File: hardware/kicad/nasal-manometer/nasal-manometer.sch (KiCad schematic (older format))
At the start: 12 parts, among them J1 Vout, J2 Vref

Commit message: Schematic updated
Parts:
- R2, R3: footprint (none) -> Resistor_SMD:R_0805_2012Metric
- Rg: footprint (none) -> Resistor_SMD:R_0603_1608Metric
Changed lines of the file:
@@
 $EndComp
 $Comp
-L power:GND #PWR?
+L power:GND #PWR0101
 U 1 1 5CD492E7
 P 5850 3725
-F 0 "#PWR?" H 5850 3475 50  0001 C CNN
+F 0 "#PWR0101" H 5850 3475 50  0001 C CNN
 F 1 "GND" H 5855 3552 50  0000 C CNN
 F 2 "" H 5850 3725 50  0001 C CNN
@@
 $EndComp
 $Comp
-L power:GND #PWR?
+L power:GND #PWR0102
 U 1 1 5CD4A19E
 P 4525 2825
-F 0 "#PWR?" H 4525 2575 50  0001 C CNN
+F 0 "#PWR0102" H 4525 2575 50  0001 C CNN
 F 1 "GND" H 4530 2652 50  0000 C CNN
 F 2 "" H 4525 2825 50  0001 C CNN
@@
 $EndComp
 $Comp
-L power:+5V #PWR?
+L power:+5V #PWR0103
 U 1 1 5CD4A7C1
 P 4525 2225
-F 0 "#PWR?" H 4525 2075 50  0001 C CNN
+F 0 "#PWR0103" H 4525 2075 50  0001 C CNN
 F 1 "+5V" H 4540 2398 50  0000 C CNN
 F 2 "" H 4525 2225 50  0001 C CNN
@@
 $EndComp
 $Comp
-L power:GND #PWR?
+L power:GND #PWR0104
 U 1 1 5CD5646F
 P 3650 2725
-F 0 "#PWR?" H 3650 2475 50  0001 C CNN
+F 0 "#PWR0104" H 3650 2475 50  0001 C CNN
 F 1 "GND" H 3655 2552 50  0000 C CNN
 F 2 "" H 3650 2725 50  0001 C CNN
@@
 $EndComp
 $Comp
-L power:GND #PWR?
+L power:GND #PWR0105
 U 1 1 5CD56C7C
 P 3900 2725
-F 0 "#PWR?" H 3900 2475 50  0001 C CNN
+F 0 "#PWR0105" H 3900 2475 50  0001 C CNN
 F 1 "GND" H 3905 2552 50  0000 C CNN
 F 2 "" H 3900 2725 50  0001 C CNN
@@
 Connection ~ 3650 2425
 $Comp
-L power:+5V #PWR?
+L power:+5V #PWR0106
 U 1 1 5CD5BB98
 P 3650 2025
-F 0 "#PWR?" H 3650 1875 50  0001 C CNN
+F 0 "#PWR0106" H 3650 1875 50  0001 C CNN
 F 1 "+5V" H 3665 2198 50  0000 C CNN
 F 2 "" H 3650 2025 50  0001 C CNN
@@
 F 0 "R2" H 4270 4321 50  0000 L CNN
 F 1 "10 KOhm" H 4270 4230 50  0000 L CNN
-F 2 "" V 4130 4275 50  0001 C CNN
+F 2 "Resistor_SMD:R_0805_2012Metric" V 4130 4275 50  0001 C CNN
 F 3 "~" H 4200 4275 50  0001 C CNN
 	1    4200 4275
@@
 F 0 "R3" H 4270 5021 50  0000 L CNN
 F 1 "15 KOhm" H 4270 4930 50  0000 L CNN
-F 2 "" V 4130 4975 50  0001 C CNN
+F 2 "Resistor_SMD:R_0805_2012Metric" V 4130 4975 50  0001 C CNN
 F 3 "~" H 4200 4975 50  0001 C CNN
 	1    4200 4975
@@
 	4200 2425 4325 2425
 $Comp
-L power:GND #PWR?
+L power:GND #PWR0107
 U 1 1 5CD3B5F1
 P 4200 5125
-F 0 "#PWR?" H 4200 4875 50  0001 C CNN
+F 0 "#PWR0107" H 4200 4875 50  0001 C CNN
 F 1 "GND" H 4205 4952 50  0000 C CNN
 F 2 "" H 4200 5125 50  0001 C CNN
@@
 	4200 4650 4200 4825
 $Comp
-L power:GND #PWR?
+L power:GND #PWR0108
 U 1 1 5CD3F60A
 P 4950 5050
-F 0 "#PWR?" H 4950 4800 50  0001 C CNN
+F 0 "#PWR0108" H 4950 4800 50  0001 C CNN
 F 1 "GND" H 4955 4877 50  0000 C CNN
 F 2 "" H 4950 5050 50  0001 C CNN
@@
 	5350 5325 5350 4750
 $Comp
-L power:+5V #PWR?
+L power:+5V #PWR0109
 U 1 1 5CD41D10
 P 4950 4450
-F 0 "#PWR?" H 4950 4300 50  0001 C CNN
+F 0 "#PWR0109" H 4950 4300 50  0001 C CNN
 F 1 "+5V" H 4965 4623 50  0000 C CNN
 F 2 "" H 4950 4450 50  0001 C CNN
@@
 Connection ~ 5350 4750
 $Comp
-L power:GND #PWR?
+L power:GND #PWR0110
 U 1 1 5CD4D2C8
 P 7125 4525
-F 0 "#PWR?" H 7125 4275 50  0001 C CNN
+F 0 "#PWR0110" H 7125 4275 50  0001 C CNN
 F 1 "GND" H 7130 4352 50  0000 C CNN
 F 2 "" H 7125 4525 50  0001 C CNN
@@
 $EndComp
 $Comp
-L power:+5V #PWR?
+L power:+5V #PWR0111
 U 1 1 5CD4D986
 P 7125 3925
-F 0 "#PWR?" H 7125 3775 50  0001 C CNN
+F 0 "#PWR0111" H 7125 3775 50  0001 C CNN
 F 1 "+5V" H 7140 4098 50  0000 C CNN
 F 2 "" H 7125 3925 50  0001 C CNN
@@
 F 0 "Rg" H 6600 4275 50  0000 L CNN
 F 1 "500 Ohm" H 6350 4175 50  0000 L CNN
-F 2 "" V 6680 4225 50  0001 C CNN
+F 2 "Resistor_SMD:R_0603_1608Metric" V 6680 4225 50  0001 C CNN
 F 3 "~" H 6750 4225 50  0001 C CNN
 	1    6750 4225

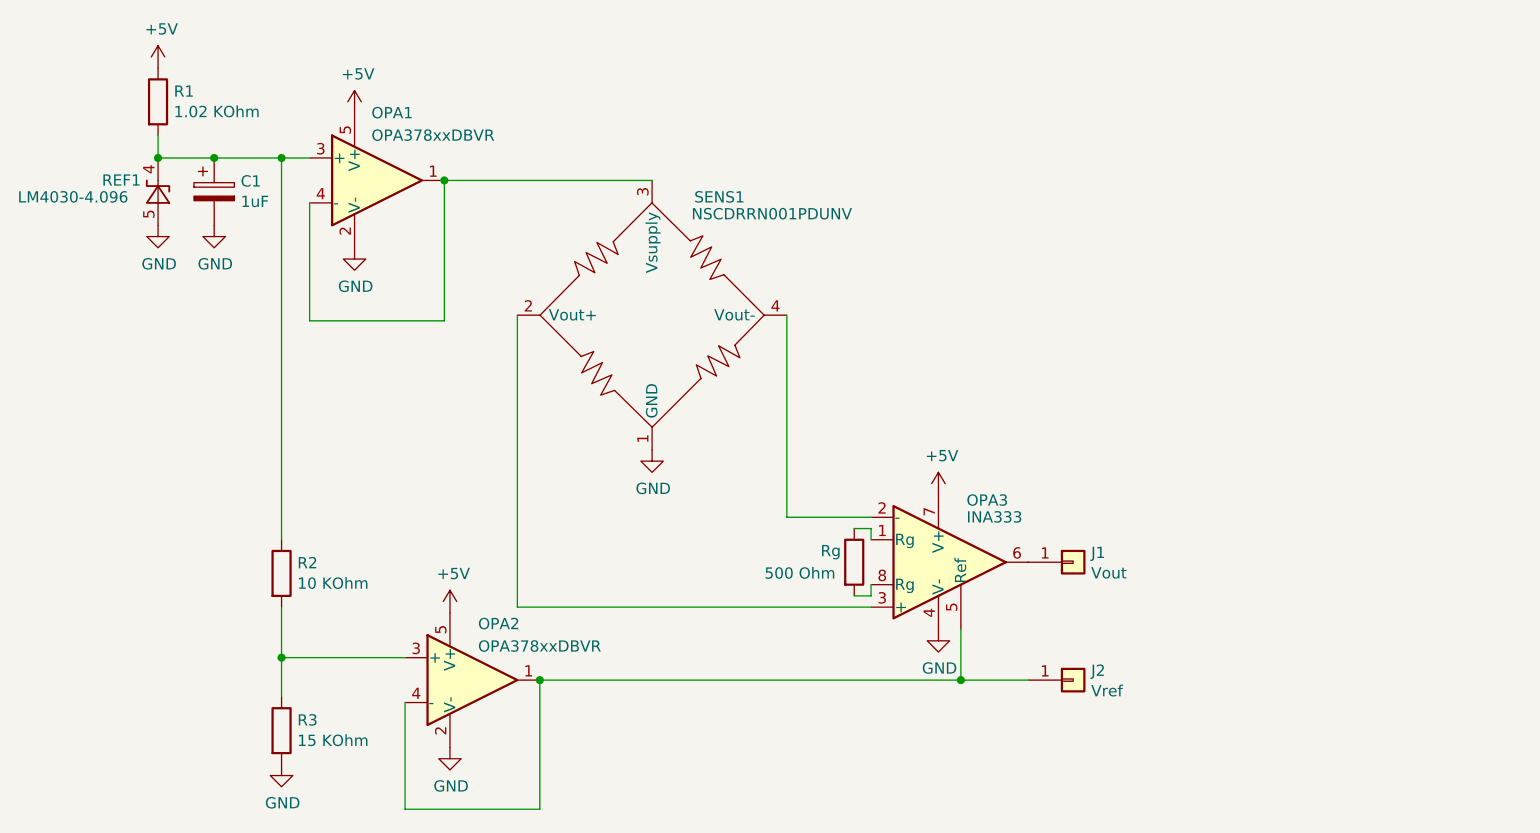
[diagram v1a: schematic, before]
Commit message: Building the board
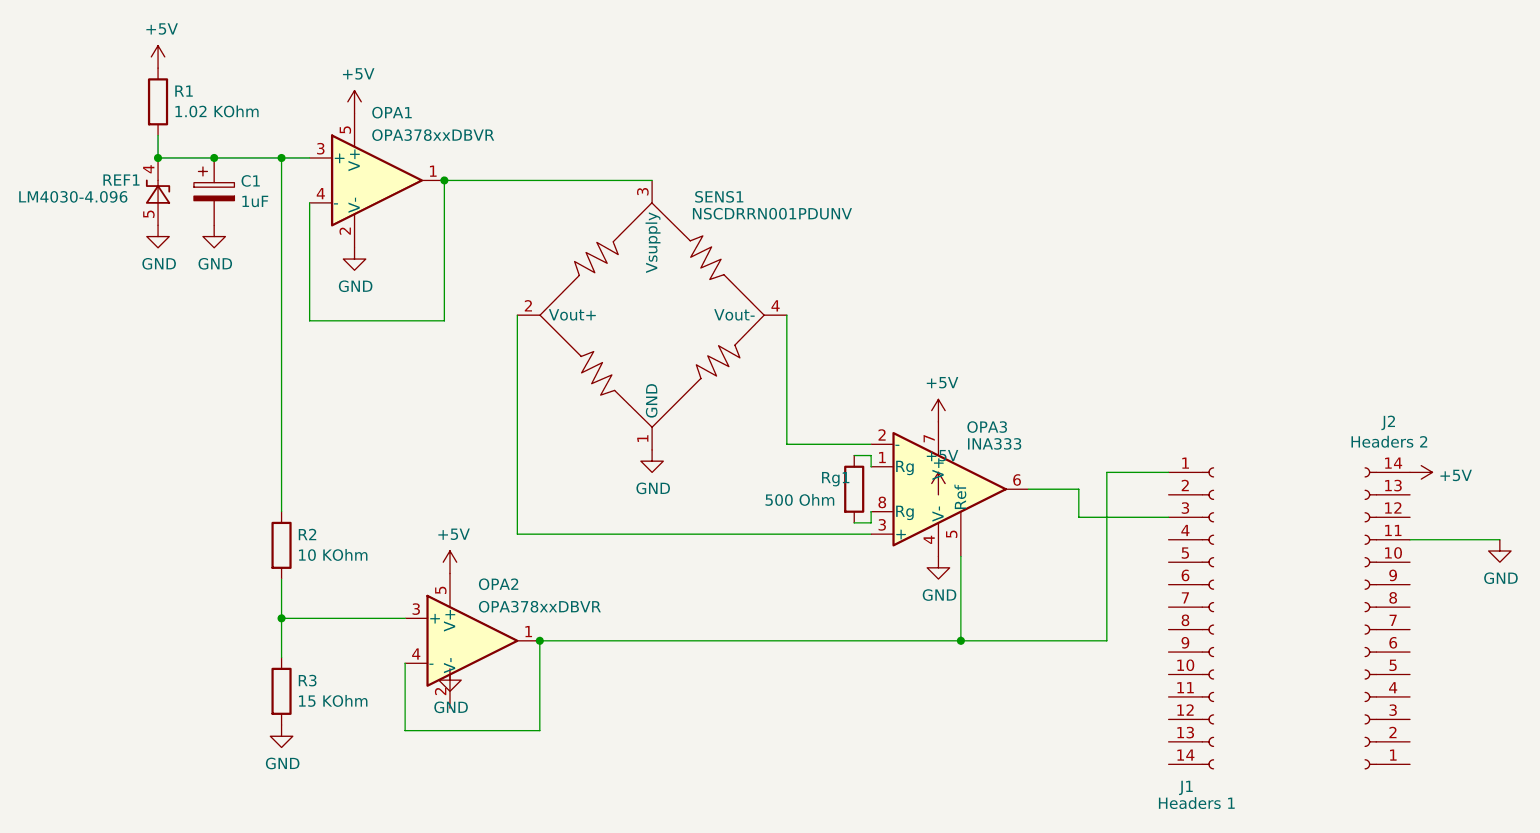
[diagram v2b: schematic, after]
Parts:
- removed J1: Vout, symbol Connector_Generic:Conn_01x01
- removed J2: Vref, symbol Connector_Generic:Conn_01x01
- added J1: Headers 1, Connector_PinSocket_2.54mm:PinSocket_1x14_P2.54mm_Vertical, symbol Connector:Conn_01x14_Female
- added J2: Headers 2, Connector_PinSocket_2.54mm:PinSocket_1x14_P2.54mm_Vertical, symbol Connector:Conn_01x14_Female
- renumbered Rg to Rg1
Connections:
- net +5V: now also J2.14 (Pin_14)
- net GND: now also J2.11 (Pin_11); no longer OPA2.2 (V-)
- net at OPA2.1, OPA2.4 (-), OPA3.5 (Ref): now also J1.1 (Pin_1)
- net at OPA3.6: now also J1.3 (Pin_3)
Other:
- moved on the sheet: OPA2, OPA3, R2, R3, Rg1
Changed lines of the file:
@@
 L Device:R R2
 U 1 1 5CD37D29
-P 4200 4275
-F 0 "R2" H 4270 4321 50  0000 L CNN
-F 1 "10 KOhm" H 4270 4230 50  0000 L CNN
-F 2 "Resistor_SMD:R_0805_2012Metric" V 4130 4275 50  0001 C CNN
-F 3 "~" H 4200 4275 50  0001 C CNN
-	1    4200 4275
+P 4200 4150
+F 0 "R2" H 4270 4196 50  0000 L CNN
+F 1 "10 KOhm" H 4270 4105 50  0000 L CNN
+F 2 "Resistor_SMD:R_0805_2012Metric" V 4130 4150 50  0001 C CNN
+F 3 "~" H 4200 4150 50  0001 C CNN
+	1    4200 4150
 	1    0    0    -1
 $EndComp
@@
 L Device:R R3
 U 1 1 5CD388C6
-P 4200 4975
-F 0 "R3" H 4270 5021 50  0000 L CNN
-F 1 "15 KOhm" H 4270 4930 50  0000 L CNN
-F 2 "Resistor_SMD:R_0805_2012Metric" V 4130 4975 50  0001 C CNN
-F 3 "~" H 4200 4975 50  0001 C CNN
-	1    4200 4975
-	1    0    0    -1
-$EndComp
-Wire Wire Line
-	3900 2425 4200 2425
-Connection ~ 4200 2425
-Wire Wire Line
-	4200 2425 4325 2425
+P 4200 4800
+F 0 "R3" H 4270 4846 50  0000 L CNN
+F 1 "15 KOhm" H 4270 4755 50  0000 L CNN
+F 2 "Resistor_SMD:R_0805_2012Metric" V 4130 4800 50  0001 C CNN
+F 3 "~" H 4200 4800 50  0001 C CNN
+	1    4200 4800
+	1    0    0    -1
+$EndComp
 $Comp
 L power:GND #PWR0107
 U 1 1 5CD3B5F1
-P 4200 5125
-F 0 "#PWR0107" H 4200 4875 50  0001 C CNN
-F 1 "GND" H 4205 4952 50  0000 C CNN
-F 2 "" H 4200 5125 50  0001 C CNN
-F 3 "" H 4200 5125 50  0001 C CNN
-	1    4200 5125
+P 4200 4950
+F 0 "#PWR0107" H 4200 4700 50  0001 C CNN
+F 1 "GND" H 4205 4777 50  0000 C CNN
+F 2 "" H 4200 4950 50  0001 C CNN
+F 3 "" H 4200 4950 50  0001 C CNN
+	1    4200 4950
 	1    0    0    -1
 $EndComp
@@
 L project_components:OPA378xxDBVR OPA2
 U 1 1 5CD3C231
-P 5050 4750
-F 0 "OPA2" H 5075 5000 50  0000 L CNN
-F 1 "OPA378xxDBVR" H 5075 4900 50  0000 L CNN
-F 2 "Package_TO_SOT_SMD:SOT-23-5" H 4950 4550 50  0001 L CNN
-F 3 "http://www.ti.com/lit/ds/symlink/opa378.pdf" H 5050 4950 50  0001 C CNN
-	1    5050 4750
-	1    0    0    -1
-$EndComp
-Wire Wire Line
-	4200 4125 4200 2425
-Wire Wire Line
-	4200 4425 4200 4650
-Wire Wire Line
-	4750 4650 4200 4650
-Connection ~ 4200 4650
-Wire Wire Line
-	4200 4650 4200 4825
+P 5050 4575
+F 0 "OPA2" H 5075 4825 50  0000 L CNN
+F 1 "OPA378xxDBVR" H 5075 4725 50  0000 L CNN
+F 2 "Package_TO_SOT_SMD:SOT-23-5" H 4950 4375 50  0001 L CNN
+F 3 "http://www.ti.com/lit/ds/symlink/opa378.pdf" H 5050 4775 50  0001 C CNN
+	1    5050 4575
+	1    0    0    -1
+$EndComp
+Connection ~ 4200 4475
+Wire Wire Line
+	4200 4475 4200 4650
 $Comp
 L power:GND #PWR0108
 U 1 1 5CD3F60A
-P 4950 5050
-F 0 "#PWR0108" H 4950 4800 50  0001 C CNN
-F 1 "GND" H 4955 4877 50  0000 C CNN
-F 2 "" H 4950 5050 50  0001 C CNN
-F 3 "" H 4950 5050 50  0001 C CNN
-	1    4950 5050
-	1    0    0    -1
-$EndComp
-Wire Wire Line
-	4750 4850 4750 5325
-Wire Wire Line
-	4750 5325 5350 5325
-Wire Wire Line
-	5350 5325 5350 4750
+P 4950 4700
+F 0 "#PWR0108" H 4950 4450 50  0001 C CNN
+F 1 "GND" H 4955 4527 50  0000 C CNN
+F 2 "" H 4950 4700 50  0001 C CNN
+F 3 "" H 4950 4700 50  0001 C CNN
+	1    4950 4700
+	1    0    0    -1
+$EndComp
+Wire Wire Line
+	4750 4975 5350 4975
+Wire Wire Line
+	5350 4975 5350 4575
 $Comp
 L power:+5V #PWR0109
 U 1 1 5CD41D10
-P 4950 4450
-F 0 "#PWR0109" H 4950 4300 50  0001 C CNN
-F 1 "+5V" H 4965 4623 50  0000 C CNN
-F 2 "" H 4950 4450 50  0001 C CNN
-F 3 "" H 4950 4450 50  0001 C CNN
-	1    4950 4450
+P 4950 4275
+F 0 "#PWR0109" H 4950 4125 50  0001 C CNN
+F 1 "+5V" H 4965 4448 50  0000 C CNN
+F 2 "" H 4950 4275 50  0001 C CNN
+F 3 "" H 4950 4275 50  0001 C CNN
+	1    4950 4275
 	1    0    0    -1
 $EndComp
@@
 L project_components:INA333 OPA3
 U 1 1 5CD4ABF9
-P 7125 4225
-F 0 "OPA3" H 7250 4500 50  0000 L CNN
-F 1 "INA333" H 7250 4425 50  0000 L CNN
-F 2 "Package_SO:VSSOP-8_3.0x3.0mm_P0.65mm" H 7225 4225 50  0001 C CNN
-F 3 "http://www.ti.com/lit/ds/symlink/ina333.pdf" H 7225 4225 50  0001 C CNN
-	1    7125 4225
-	1    0    0    -1
-$EndComp
-Wire Wire Line
-	5250 3125 5250 4425
-Wire Wire Line
-	5250 4425 6825 4425
-Wire Wire Line
-	6450 3125 6450 4025
-Wire Wire Line
-	6450 4025 6825 4025
-Wire Wire Line
-	5350 4750 7225 4750
-Wire Wire Line
-	7225 4750 7225 4525
-Connection ~ 5350 4750
+P 7125 3900
+F 0 "OPA3" H 7250 4175 50  0000 L CNN
+F 1 "INA333" H 7250 4100 50  0000 L CNN
+F 2 "Package_SO:VSSOP-8_3.0x3.0mm_P0.65mm" H 7225 3900 50  0001 C CNN
+F 3 "http://www.ti.com/lit/ds/symlink/ina333.pdf" H 7225 3900 50  0001 C CNN
+	1    7125 3900
+	1    0    0    -1
+$EndComp
+Wire Wire Line
+	5250 4100 6825 4100
+Wire Wire Line
+	5350 4575 7225 4575
 $Comp
 L power:GND #PWR0110
 U 1 1 5CD4D2C8
-P 7125 4525
-F 0 "#PWR0110" H 7125 4275 50  0001 C CNN
-F 1 "GND" H 7130 4352 50  0000 C CNN
-F 2 "" H 7125 4525 50  0001 C CNN
-F 3 "" H 7125 4525 50  0001 C CNN
-	1    7125 4525
+P 7125 4200
+F 0 "#PWR0110" H 7125 3950 50  0001 C CNN
+F 1 "GND" H 7130 4027 50  0000 C CNN
+F 2 "" H 7125 4200 50  0001 C CNN
+F 3 "" H 7125 4200 50  0001 C CNN
+	1    7125 4200
 	1    0    0    -1
 $EndComp
@@
 $EndComp
 $Comp
-L Device:R Rg
+L Device:R Rg1
 U 1 1 5CD4E01B
-P 6750 4225
-F 0 "Rg" H 6600 4275 50  0000 L CNN
-F 1 "500 Ohm" H 6350 4175 50  0000 L CNN
-F 2 "Resistor_SMD:R_0603_1608Metric" V 6680 4225 50  0001 C CNN
-F 3 "~" H 6750 4225 50  0001 C CNN
-	1    6750 4225
-	1    0    0    -1
-$EndComp
-Wire Wire Line
-	6825 4075 6825 4125
-Wire Wire Line
-	6825 4375 6825 4325
-Wire Wire Line
-	6750 4075 6825 4075
-Wire Wire Line
-	6750 4375 6825 4375
-$Comp
-L Connector_Generic:Conn_01x01 J1
-U 1 1 5CD5713A
-P 7725 4225
-F 0 "J1" H 7805 4267 50  0000 L CNN
-F 1 "Vout" H 7805 4176 50  0000 L CNN
-F 2 "" H 7725 4225 50  0001 C CNN
-F 3 "~" H 7725 4225 50  0001 C CNN
-	1    7725 4225
-	1    0    0    -1
-$EndComp
-$Comp
-L Connector_Generic:Conn_01x01 J2
-U 1 1 5CD583A8
-P 7725 4750
-F 0 "J2" H 7805 4792 50  0000 L CNN
-F 1 "Vref" H 7805 4701 50  0000 L CNN
-F 2 "" H 7725 4750 50  0001 C CNN
-F 3 "~" H 7725 4750 50  0001 C CNN
-	1    7725 4750
-	1    0    0    -1
-$EndComp
-Wire Wire Line
-	7225 4750 7525 4750
-Connection ~ 7225 4750
+P 6750 3900
+F 0 "Rg1" H 6600 3950 50  0000 L CNN
+F 1 "500 Ohm" H 6350 3850 50  0000 L CNN
+F 2 "Resistor_SMD:R_0603_1608Metric" V 6680 3900 50  0001 C CNN
+F 3 "~" H 6750 3900 50  0001 C CNN
+	1    6750 3900
+	1    0    0    -1
+$EndComp
+Wire Wire Line
+	6825 3750 6825 3800
+Wire Wire Line
+	6750 3750 6825 3750
+Wire Wire Line
+	6750 4050 6825 4050
+$Comp
+L Connector:Conn_01x14_Female J1
+U 1 1 5CD7F223
+P 8350 4425
+F 0 "J1" H 8200 3625 50  0000 L CNN
+F 1 "Headers 1" H 8100 3550 50  0000 L CNN
+F 2 "Connector_PinSocket_2.54mm:PinSocket_1x14_P2.54mm_Vertical" H 8350 4425 50  0001 C CNN
+F 3 "~" H 8350 4425 50  0001 C CNN
+	1    8350 4425
+	1    0    0    -1
+$EndComp
+$Comp
+L Connector:Conn_01x14_Female J2
+U 1 1 5CD8CCB6
+P 9025 4525
+F 0 "J2" H 8917 3600 50  0000 C CNN
+F 1 "Headers 2" H 8917 3691 50  0000 C CNN
+F 2 "Connector_PinSocket_2.54mm:PinSocket_1x14_P2.54mm_Vertical" H 9025 4525 50  0001 C CNN
+F 3 "~" H 9025 4525 50  0001 C CNN
+	1    9025 4525
+	-1   0    0    1
+$EndComp
+Connection ~ 5350 4575
+Wire Wire Line
+	4750 4675 4750 4975
+Wire Wire Line
+	4750 4475 4200 4475
+Wire Wire Line
+	4200 4300 4200 4475
+Wire Wire Line
+	5250 3125 5250 4100
+Wire Wire Line
+	6825 4000 6825 4050
+Wire Wire Line
+	6825 3700 6450 3700
+Wire Wire Line
+	6450 3700 6450 3125
+Wire Wire Line
+	3900 2425 4200 2425
+Wire Wire Line
+	4200 4000 4200 2425
+Connection ~ 4200 2425
+Wire Wire Line
+	4200 2425 4325 2425
+Wire Wire Line
+	7225 4200 7225 4575
+Wire Wire Line
+	7225 4575 7875 4575
+Wire Wire Line
+	7875 4575 7875 3825
+Wire Wire Line
+	7875 3825 8150 3825
+Connection ~ 7225 4575
+Wire Wire Line
+	7525 3900 7750 3900
+Wire Wire Line
+	7750 3900 7750 4025
+Wire Wire Line
+	7750 4025 8150 4025
+$Comp
+L power:+5V #PWR0112
+U 1 1 5CDA9387
+P 9225 3825
+F 0 "#PWR0112" H 9225 3675 50  0001 C CNN
+F 1 "+5V" V 9240 3953 50  0000 L CNN
+F 2 "" H 9225 3825 50  0001 C CNN
+F 3 "" H 9225 3825 50  0001 C CNN
+	1    9225 3825
+	0    1    1    0
+$EndComp
+$Comp
+L power:GND #PWR0113
+U 1 1 5CDAA912
+P 9625 4125
+F 0 "#PWR0113" H 9625 3875 50  0001 C CNN
+F 1 "GND" H 9630 3952 50  0000 C CNN
+F 2 "" H 9625 4125 50  0001 C CNN
+F 3 "" H 9625 4125 50  0001 C CNN
+	1    9625 4125
+	1    0    0    -1
+$EndComp
+Wire Wire Line
+	9225 4125 9625 4125
+$Comp
+L power:+5V #PWR?
+U 1 1 5CDB8638
+P 7125 3600
+F 0 "#PWR?" H 7125 3450 50  0001 C CNN
+F 1 "+5V" H 7140 3773 50  0000 C CNN
+F 2 "" H 7125 3600 50  0001 C CNN
+F 3 "" H 7125 3600 50  0001 C CNN
+	1    7125 3600
+	1    0    0    -1
+$EndComp
 $EndSCHEMATC
